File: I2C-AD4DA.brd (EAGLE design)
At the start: 50 x 50 mm, 17 parts, among them IC1 PCF8591T, X1 RJ45-FRONT

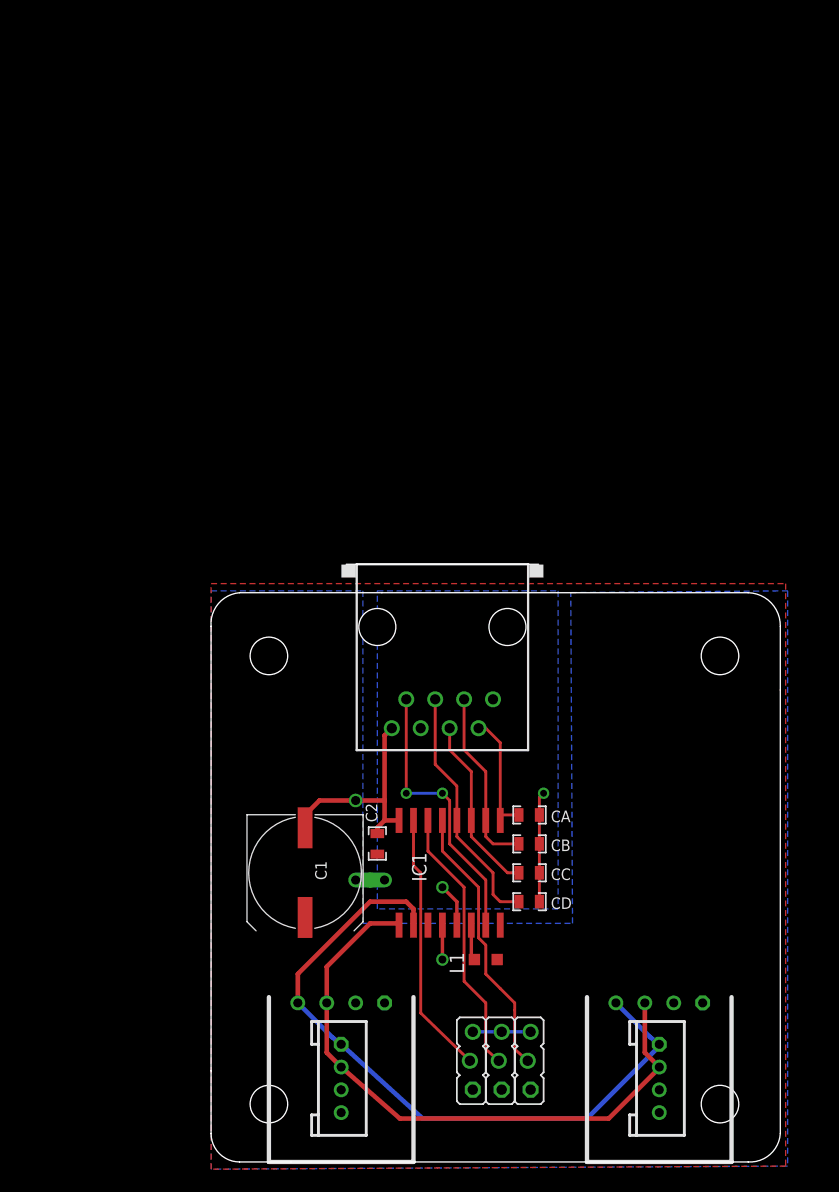
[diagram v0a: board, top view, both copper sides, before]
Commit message: 2.0
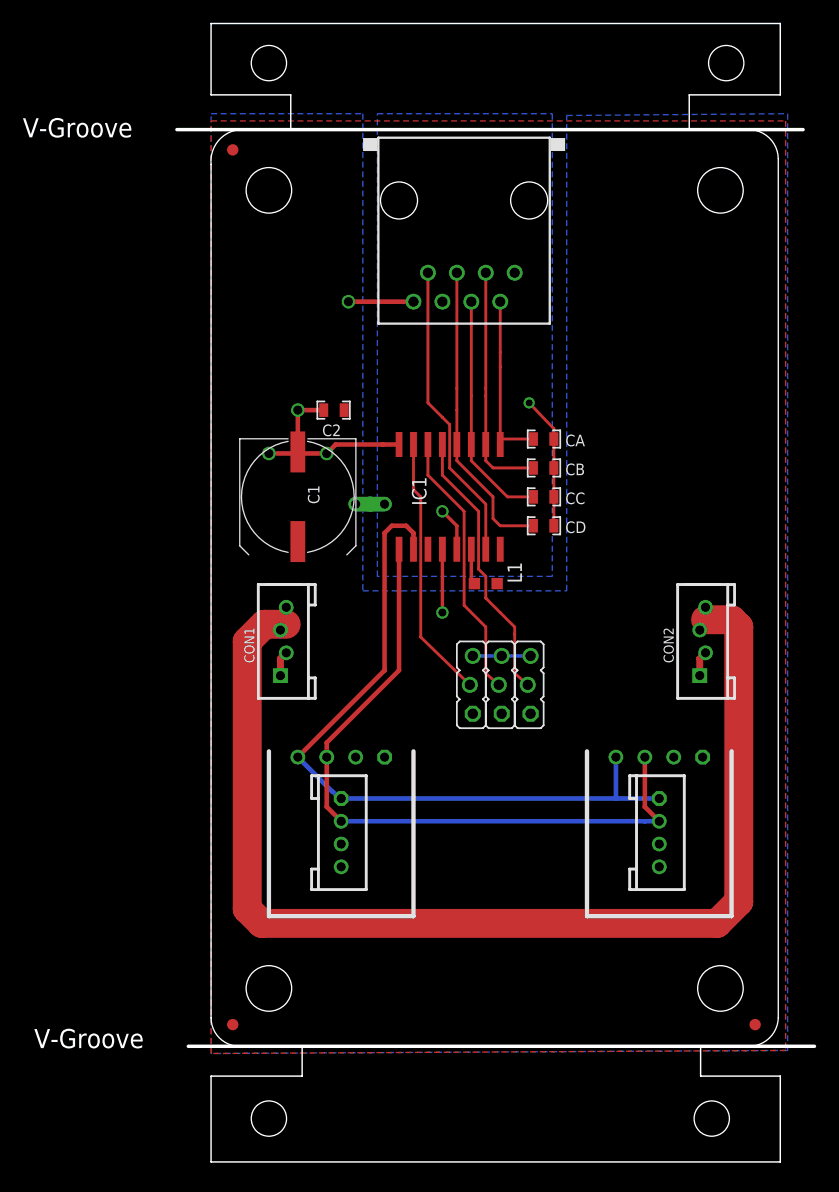
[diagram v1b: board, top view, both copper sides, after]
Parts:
- removed U$9: BOARD50X50, SPCoast-minimal:BOARD-SEEED5X5
- added BOARD1: (no value), SPCoast:BOARD-DINRAIL-3.17INX5CM
- added CON1, CON2: CONNECTOR-GROVE-4P-2.0-3470130P1, SPCoast:4P-2.0
- A0, A1, A2: device SPCoast-minimal:J3-254 -> SPCoast:J3-254
- IC1: device micro-philips:SO16W -> SPCoast:SO16W
- L1: device rcl:L2012C -> SPCoast:L2012C
- LOGO1: value OSHW-LOGOL -> DOC-OSHW-LOGO-L; device SPCoast-minimal:OSHW-LOGO-L -> SPCoast:OSHW-LOGO-L
- X1: value RJ45-FRONT -> (none); device SPCoast-minimal:RJ45-NO-SHIELD -> SPCoast:RJ45-NO-SHIELD
- moved C2 38.3 mm to (10.8, 66.0), turned to 180 degrees
- moved X1 37.5 mm to (22.2, 84.5)
- moved LOGO1 33.1 mm to (7.62, 77.5)
- moved CC 33.0 mm to (29.2, 58.4)
- moved CD 33.0 mm to (29.2, 55.9)
- moved CA 33.0 mm to (29.2, 63.5)
- moved CB 33.0 mm to (29.2, 61.0)
- moved C1 33.0 mm to (7.62, 58.4)
- moved IC1 33.0 mm to (21.0, 58.4)
- moved A0 33.0 mm to (27.9, 41.9)
- moved A1 33.0 mm to (25.4, 41.9)
- moved A2 33.0 mm to (22.9, 41.9)
- moved L1 33.0 mm to (24.1, 50.8)
- moved U$1 33.0 mm to (14.0, 57.8)
- moved I2C0 21.6 mm to (11.4, 35.6)
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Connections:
- new net VIN: CON1.3, CON1.4, CON2.3, CON2.4
- net GND: now also CON1.1, CON1.2, CON2.1, CON2.2
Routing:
- net VIN: track 0.00 -> 103.8 mm
- net GND: track 23.2 -> 34.1 mm, vias 2 -> 5
- net SDA: track 55.1 -> 61.2 mm
- net AD1: track 16.0 -> 21.0 mm
- net AD3: track 21.8 -> 26.7 mm
- net AD2: track 15.8 -> 20.7 mm
- net AD0: track 11.4 -> 15.9 mm
- net SCL: track 60.8 -> 64.2 mm
- net AGND: track 13.5 -> 15.5 mm
- net DA0: track 24.6 -> 26.4 mm, vias 2 -> 0
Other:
- board size 50 x 50 mm -> 56 x 100 mm
- board text added: "2018-07"
- board text added: "I2C-AD4DA"
- board text added: "Vin"
- board text added: "v2.0"
- board text removed: "2014-10"
- board text removed: "2014-12"
- board text removed: "v1.1"
